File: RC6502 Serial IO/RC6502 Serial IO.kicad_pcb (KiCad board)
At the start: 2 copper layers, 99.1 x 66 mm, 16 parts, among them J1 CONN_01X39, J2 Arduino Nano, J3 SPI Breakout, SW1 Reset, U1 74HCT04, U2 WD65C21, U3 74LS138, U4 MCP23S17

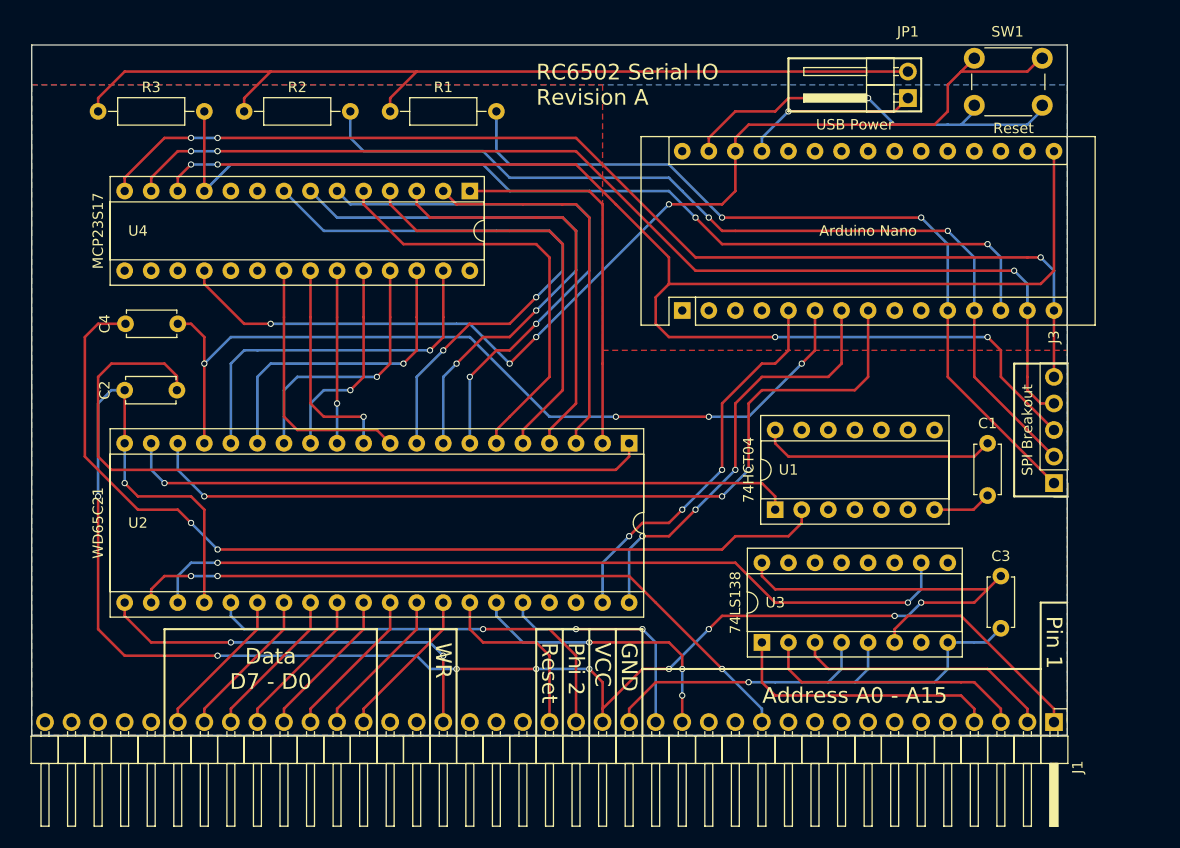
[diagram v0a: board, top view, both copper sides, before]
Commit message: Serial IO Revision B
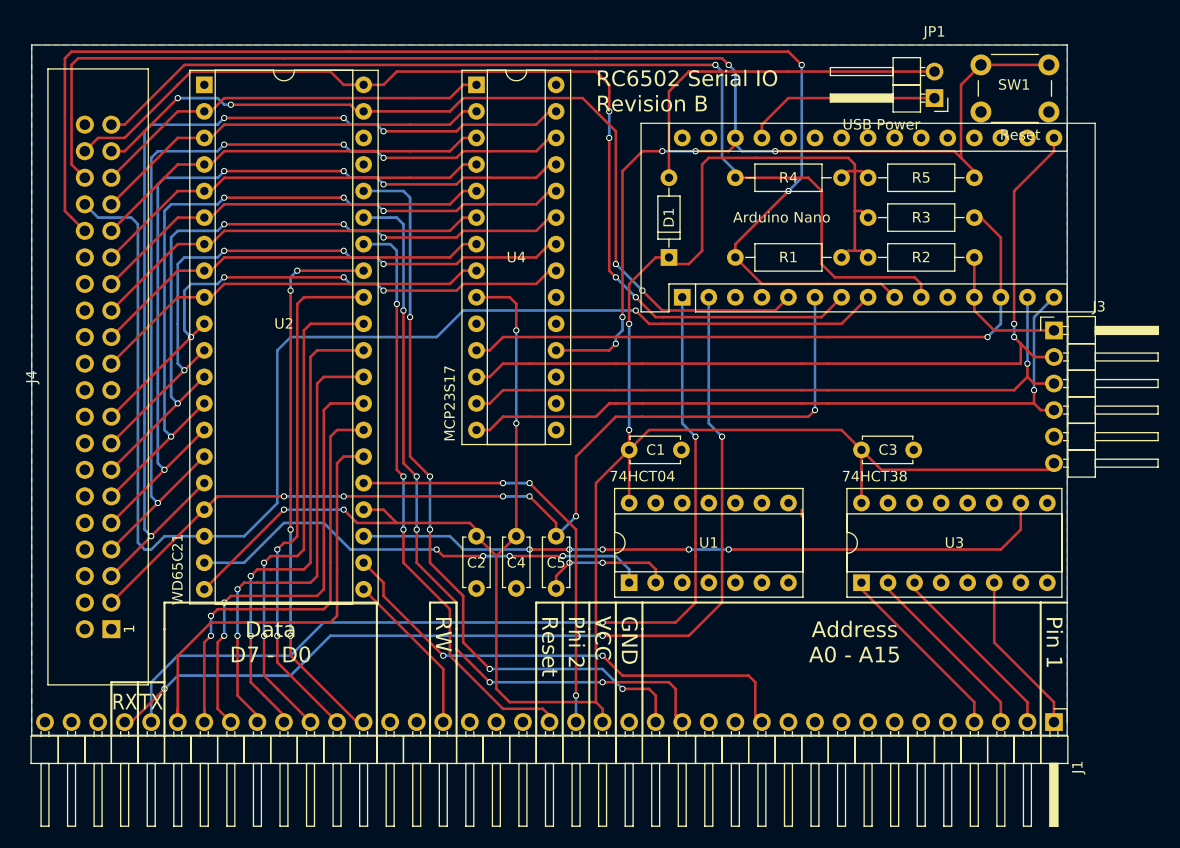
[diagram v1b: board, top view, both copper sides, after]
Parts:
- added C5: 10nF, Capacitors_THT:C_Disc_D4.7mm_W2.5mm_P5.00mm, F.Cu at (149.2, 115.6)
- added D1: 1N4848, Diodes_THT:D_DO-35_SOD27_P7.62mm_Horizontal, F.Cu at (160.0, 88.9)
- added J4: Peripheral Bus, Connectors:IDC_Header_Straight_40pins, F.Cu at (106.7, 124.5)
- added R4: 10k, Resistors_THT:R_Axial_DIN0207_L6.3mm_D2.5mm_P10.16mm_Horizontal, F.Cu at (166.4, 81.3)
- added R5: 10k, Resistors_THT:R_Axial_DIN0207_L6.3mm_D2.5mm_P10.16mm_Horizontal, F.Cu at (189.2, 81.3)
- C4: value 10nF -> 100nF
- J3: footprint Pin_Headers:Pin_Header_Straight_1x05_Pitch2.54mm -> Pin_Headers:Pin_Header_Angled_1x06_Pitch2.54mm
- U3: value 74LS138 -> 74HCT38
- moved R3 74.4 mm to (179.1, 85.1)
- moved R2 61.3 mm to (179.1, 88.9)
- moved U2 53.2 mm to (115.6, 72.4), turned to 0 degrees
- moved C4 38.2 mm to (145.4, 115.6), turned to 270 degrees
- moved C2 36.4 mm to (141.6, 115.6), turned to 270 degrees
- moved R1 35.9 mm to (166.4, 88.9)
- moved C1 34.3 mm to (156.2, 107.3), turned to 0 degrees
- moved C3 18.0 mm to (178.4, 107.3), turned to 0 degrees
- moved U1 15.6 mm to (156.2, 120.0)
- moved J3 14.6 mm to (196.8, 95.9), turned to 0 degrees
- moved U3 11.1 mm to (178.4, 120.0)
- moved U4 10.2 mm to (141.6, 72.4), turned to 0 degrees
- moved JP1 2.54 mm to (185.4, 73.7)
- moved J2 1.27 mm to (161.3, 92.7)
- moved SW1 0.90 mm to (189.9, 70.5)
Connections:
- net KBD_DA renamed KBD_STROBE
- net Net-(J2-Pad28) renamed P_RESET
- net OUT_READY renamed OUT_RDA
- net WR renamed RW
- C4 pad 1: OUT_DA -> VCC
- C4 pad 2: Net-(C4-Pad2) -> GND
- J1 pad 35: (no net) -> TX
- J1 pad 36: (no net) -> RX
- J2 pad 1: (no net) -> TX
- J2 pad 10: (no net) -> KBD_DETECT
- J2 pad 11: /CS1 -> (no net)
- J2 pad 12: /CS2 -> /CS1
- J2 pad 2: (no net) -> RX
- J2 pad 9: (no net) -> OUT_DETECT
- J3 pad 2: /CS2 -> /SCK
- J3 pad 3: /SCK -> /MOSI
- J3 pad 4: /MOSI -> /MISO
- J3 pad 5: /MISO -> GND
- JP1 pad 2: VCC -> Net-(D1-Pad2)
- R1 pad 1: VCC -> OUT_DETECT
- R1 pad 2: /CS1 -> VCC
- R2 pad 2: /CS2 -> /CS1
- U1 pad 2: Net-(C4-Pad2) -> Net-(C5-Pad2)
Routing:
- net GND: track 165.7 -> 0.00 mm, vias 2 -> 0
- net OUT_DETECT: track 0.00 -> 126.4 mm, vias 0 -> 2
- net KBD_DETECT: track 0.00 -> 99.1 mm, vias 0 -> 1
- net RX: track 0.00 -> 91.6 mm, vias 0 -> 3
- net Net-(C4-Pad2): track 90.4 -> 0.00 mm, vias 2 -> 0
- net /CS2: track 89.2 -> 0.00 mm, vias 2 -> 0
- net TX: track 0.00 -> 88.8 mm, vias 0 -> 2
- net /SCK: track 151.9 -> 79.7 mm, vias 4 -> 2
- net /CS1: track 77.7 -> 13.5 mm, vias 2 -> 0
- net OUT_D6: track 35.3 -> 92.8 mm, vias 1 -> 4
- net KBD_STROBE: track 41.6 -> 98.2 mm, vias 3 -> 4
- net OUT_D5: track 30.3 -> 86.4 mm, vias 1 -> 4
- net P_RESET: track 102.9 -> 158.6 mm, vias 4 -> 6
- net OUT_D4: track 25.2 -> 80.1 mm, vias 1 -> 4
- net OUT_D3: track 20.1 -> 73.7 mm, vias 1 -> 4
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- removed copper zone on F.Cu, net VCC
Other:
- board text added: "RC6502 Serial IO Revision B"
- board text added: "RW"
- board text added: "RX"
- board text added: "TX"
- board text removed: "RC6502 Serial IO Revision A"
- board text removed: "WR"
